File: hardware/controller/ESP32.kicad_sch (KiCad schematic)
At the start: 1 part, among them U2 ESP32-S3

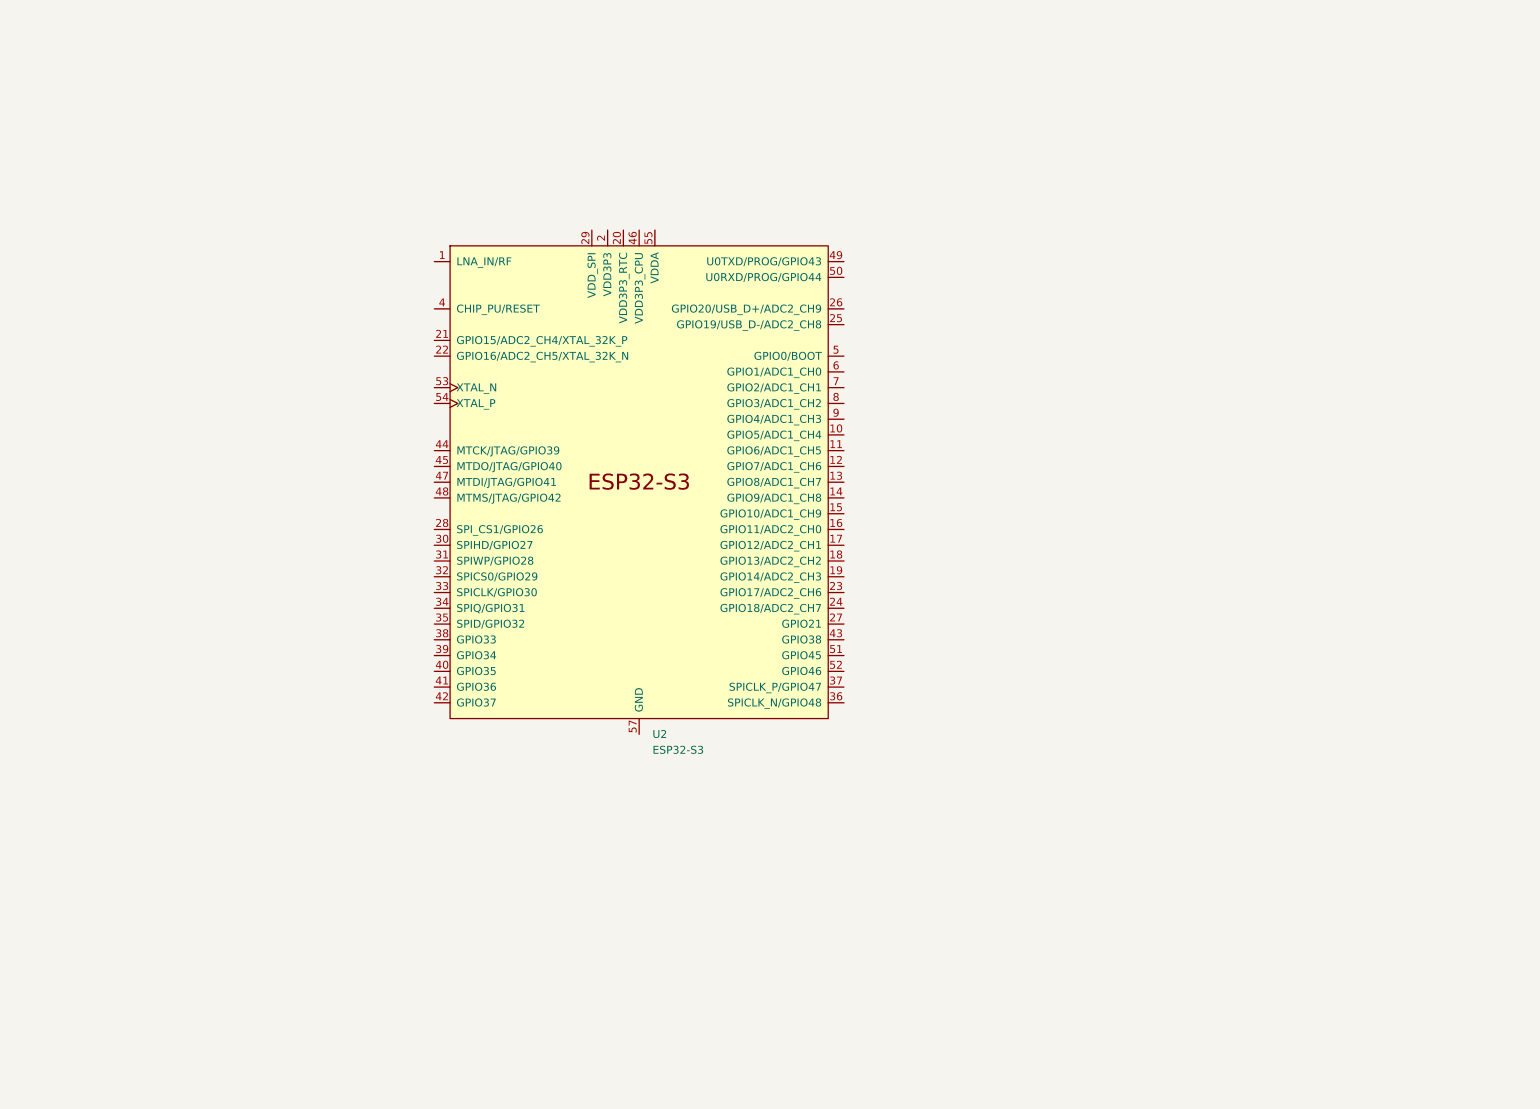
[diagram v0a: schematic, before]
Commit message: a
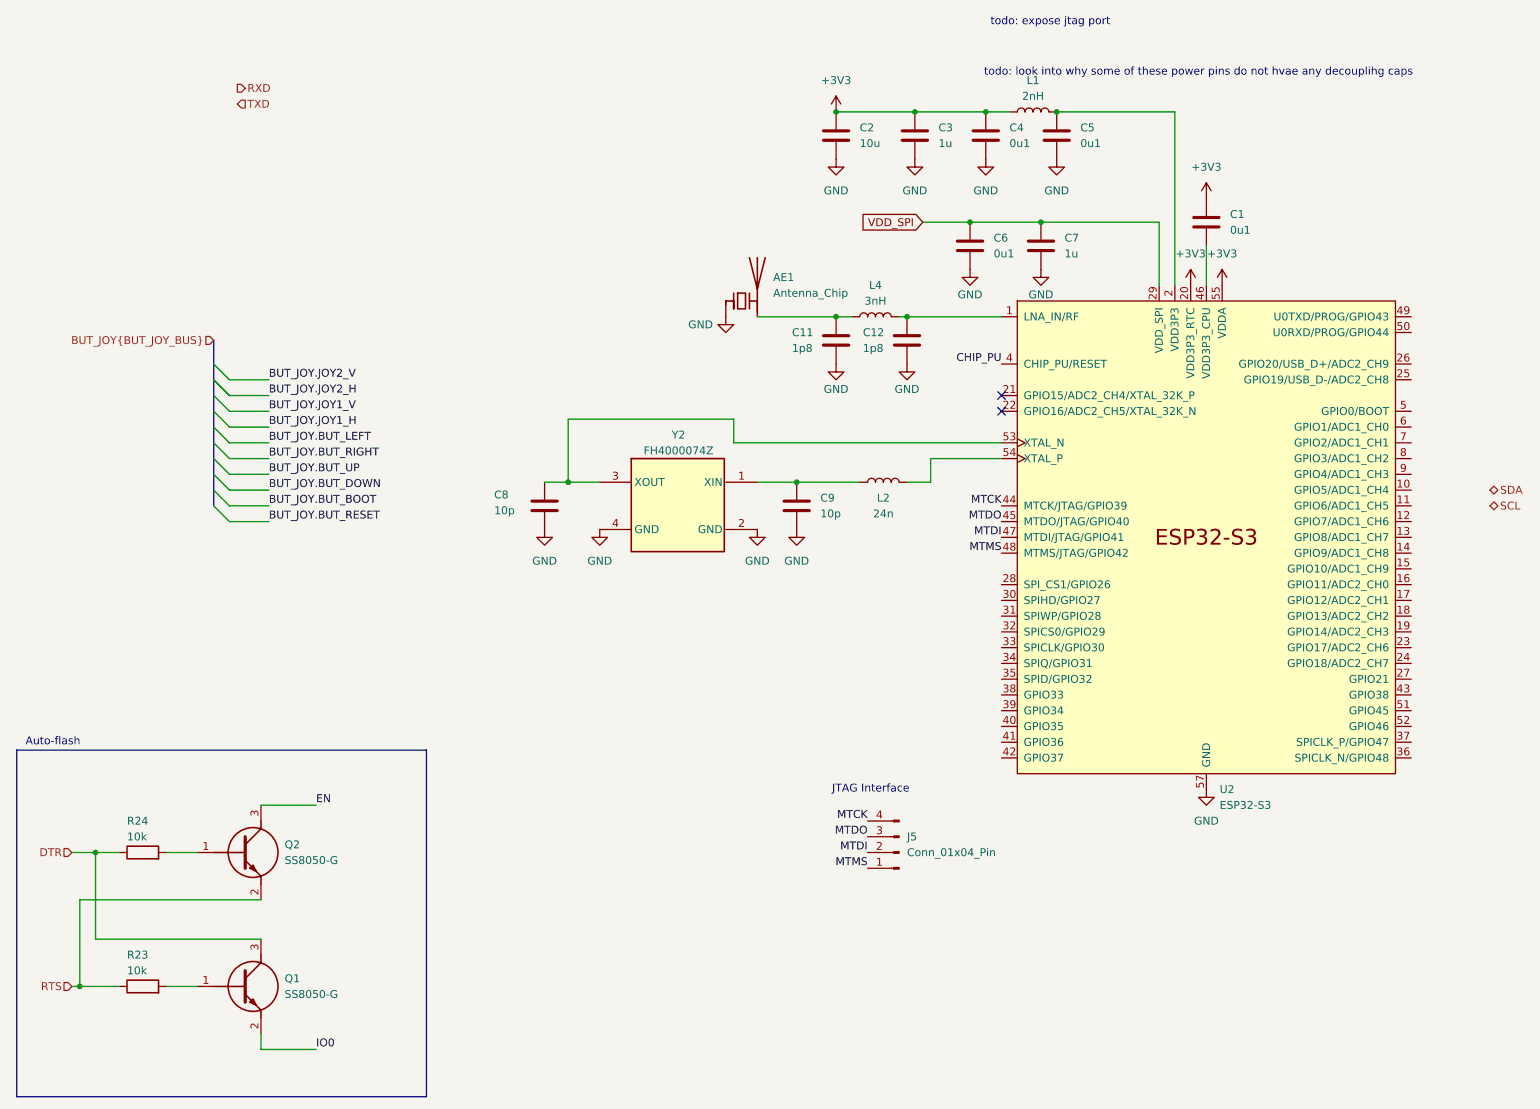
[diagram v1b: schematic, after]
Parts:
- added AE1: Antenna_Chip, symbol Device:Antenna_Chip
- added C1, C4, C5, C6: 0u1, symbol Device:C
- added C11, C12: 1p8, symbol Device:C
- added C2: 10u, symbol Device:C
- added C3, C7: 1u, symbol Device:C
- added C8, C9: 10p, symbol Device:C
- added J5: Conn_01x04_Pin, symbol Connector:Conn_01x04_Pin
- added L1: 2nH, symbol Device:L
- added L2: 24n, symbol Device:L
- added L4: 3nH, symbol Device:L
- added Q1, Q2: SS8050-G, SOT95P240X115-3N, symbol SamacSys_Parts:SS8050-G
- added R23, R24: 10k, symbol Device:R
- added Y2: FH4000074Z, FH4000074Z, symbol SamacSys_Parts:FH4000074Z
- U2: symbol Espressif:ESP32-S3 -> SamacSys_Parts:ESP32-S3
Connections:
- net VDD3P3: now also C5.1, L1.2
- net at U2.1 (LNA_IN/RF): now also C12.1, L4.2
- net +3V3: now reaches U2.20 (VDD3P3_RTC)
- net +3V3: now also U2.55 (VDDA), U2.56 (VDDA), C1.1, C2.1, C3.1, C4.1, L1.1
- net VDD_SPI: now reaches U2.29 (VDD_SPI)
- net VDD_SPI: now also C6.1, C7.1
- net CHIP_PU: now reaches U2.4 (CHIP_PU/RESET)
- net MTCK: now reaches U2.44 (MTCK/JTAG/GPIO39)
- net MTCK: now also J5.4 (Pin_4)
- net MTDO: now reaches U2.45 (MTDO/JTAG/GPIO40)
- net MTDO: now also J5.3 (Pin_3)
- net at U2.46 (VDD3P3_CPU): now also C1.2
- net MTDI: now reaches U2.47 (MTDI/JTAG/GPIO41)
- net MTDI: now also J5.2 (Pin_2)
- net MTMS: now reaches U2.48 (MTMS/JTAG/GPIO42)
- net MTMS: now also J5.1 (Pin_1)
- net at U2.53 (XTAL_N): now also C8.1, Y2.3 (XOUT)
- net at U2.54 (XTAL_P): now also L2.2
- net GND: now reaches U2.57 (GND)
- net GND: now also AE1.1 (FEED), C11.2, C12.2, C2.2, C3.2, C4.2, C5.2, C6.2, C7.2, C8.2, C9.2, Y2.2 (GND), Y2.4 (GND)
- new net: Q2.1 (B), R24.2
- new net: AE1.2 (PCB_Trace), C11.1, L4.1
- new net: C9.1, L2.1, Y2.1 (XIN)
- new net: Q1.1 (B), R23.2
- new net DTR: Q1.3 (C), R24.1
- new net EN: Q2.3 (C)
- new net IO0: Q1.2 (E)
- new net RTS: Q2.2 (E), R23.1
- no-connect marks 0 -> 2
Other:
- note added: "Auto-flash"
- note added: "JTAG Interface"
- note added: "todo: expose jtag port"
- note added: "todo: look into why some of these power pins do not hvae any decouplihg caps"
- moved on the sheet: U2
